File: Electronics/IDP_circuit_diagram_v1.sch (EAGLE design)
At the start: 33 parts, among them Q1 ARDUINOR3-NOIOREF-NOTEXT

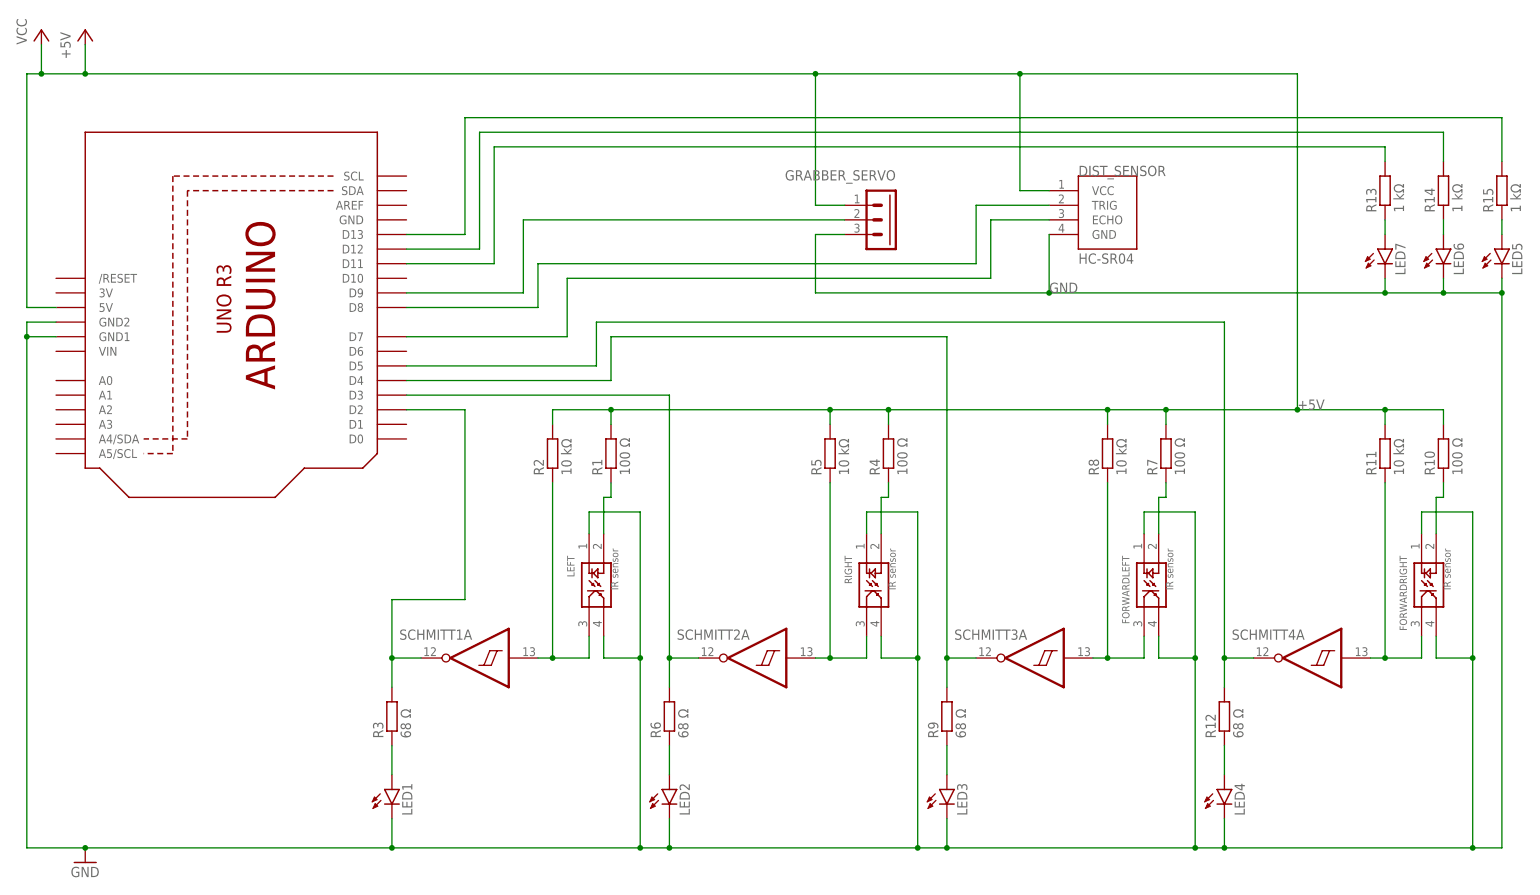
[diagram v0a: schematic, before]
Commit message: updated circuit diagram
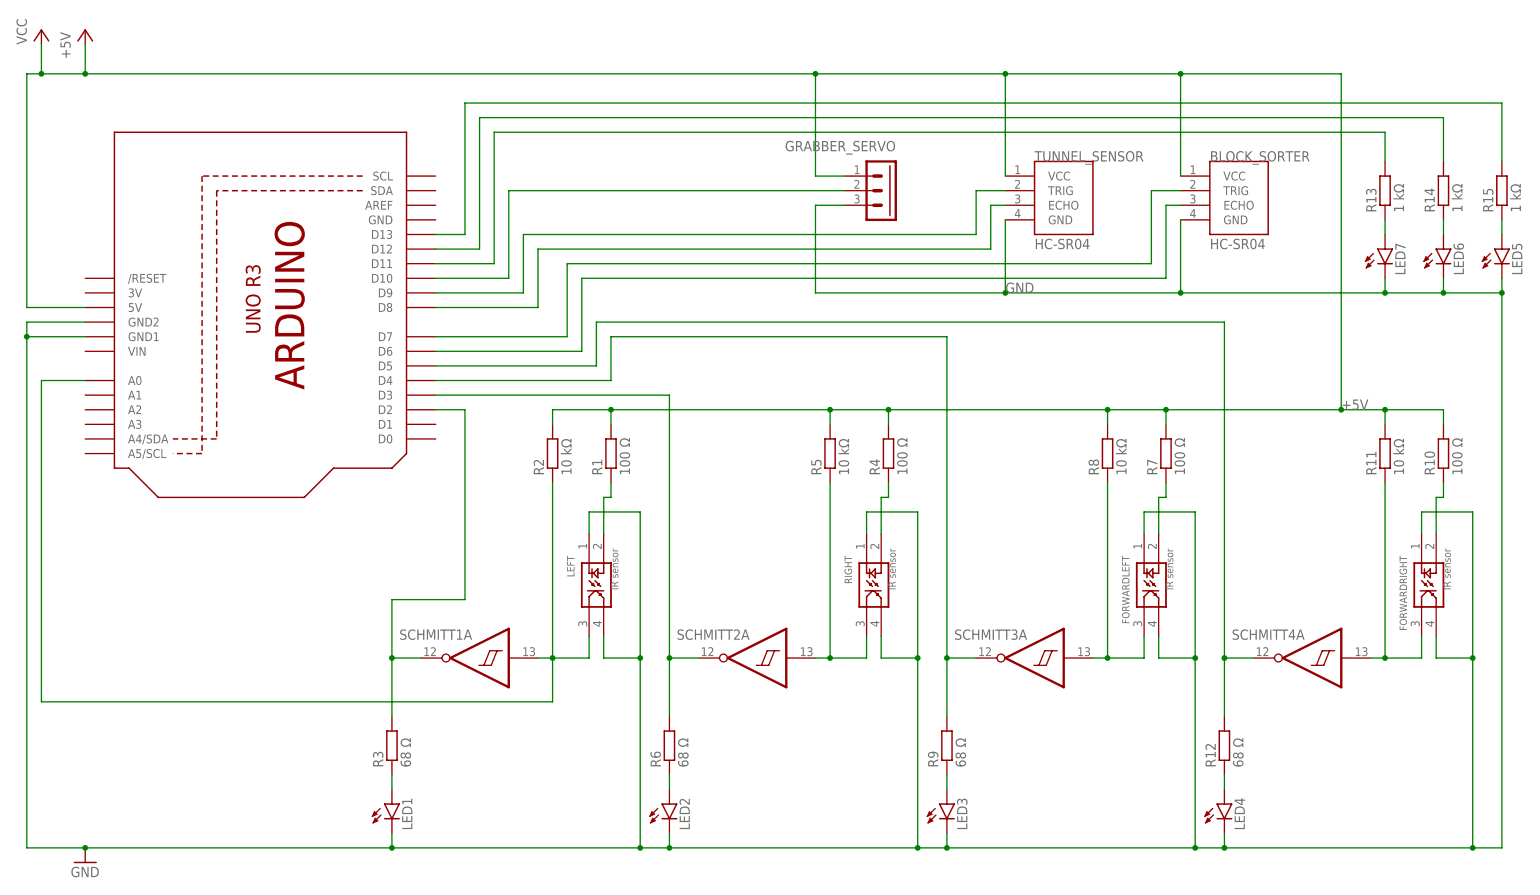
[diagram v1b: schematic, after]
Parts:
- removed DIST_SENSOR: HC-SR04, IDP_library:HC-SR04
- added BLOCK_SORTER, TUNNEL_SENSOR: HC-SR04, IDP_library:HC-SR04
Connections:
- new net N$1: BLOCK_SORTER.ECHO, Q1.D6
- new net N$3: BLOCK_SORTER.TRIG, Q1.D7
- net +5V: now also BLOCK_SORTER.VCC, TUNNEL_SENSOR.VCC; no longer DIST_SENSOR.VCC
- net GND: now also BLOCK_SORTER.GND, TUNNEL_SENSOR.GND; no longer DIST_SENSOR.GND
- net N$19: now also Q1.D10; no longer Q1.D9
- net N$20: now also Q1.D9, TUNNEL_SENSOR.TRIG; no longer DIST_SENSOR.TRIG, Q1.D8
- net N$36: now also Q1.D8, TUNNEL_SENSOR.ECHO; no longer DIST_SENSOR.ECHO, Q1.D7
- net N$57: now also Q1.A0
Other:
- moved on the sheet: GRABBER_SERVO, LED1, LED2, LED3, LED4, R12, R3, R6, R9
